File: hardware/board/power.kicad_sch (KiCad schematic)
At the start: 179 parts, among them J2 USB_C_Receptacle, Q1 WPM3407-3/TR, Q2 SS8050, Q3 WPM2015-3/TR_C7472861, U10 SY8088AAC, U12 SY7208ABC, U4 RK809-5, U6 TMUXHS4212RKSR, U7 FUSB302BMPX, U8 BQ25890RTWR, U9 S2B-PH-K-S(LF)(SN), X2 Q13FC1350000400

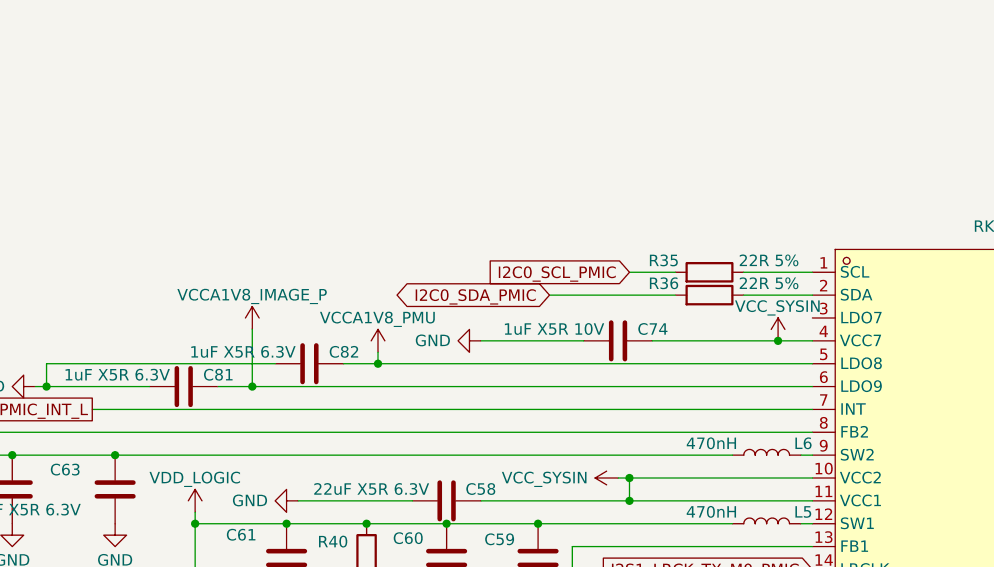
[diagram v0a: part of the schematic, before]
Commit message: revised power
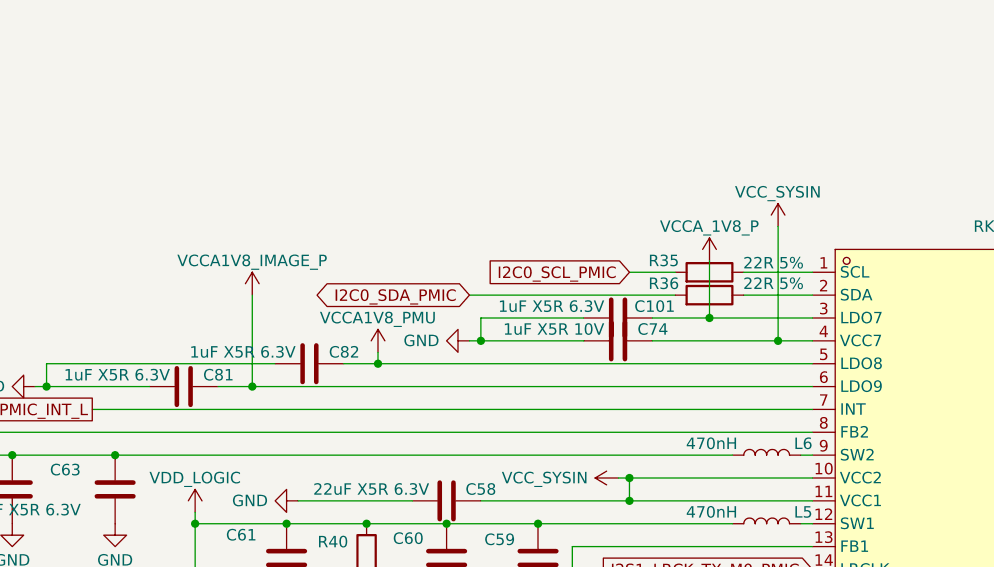
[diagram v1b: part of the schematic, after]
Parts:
- added C101: 1uF X5R 6.3V, Capacitor_SMD:C_0402_1005Metric, symbol Device:C
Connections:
- net GND: now also C101.1
- net VCCA_1V8_P: now also U4.3 (LDO7), C101.2
